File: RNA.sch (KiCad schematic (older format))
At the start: 89 parts, among them J1 USB_B_Micro, J2 AudioJack4, J3 AudioJack4, J4 Conn_01x06, SW1 SW_SPST, SW10 SW_Push_45deg, SW11 SW_Push_45deg, SW12 SW_Push_45deg, SW13 SW_Push_45deg, SW14 SW_Push_45deg, SW15 SW_Push_45deg, SW16 SW_Push_45deg, SW17 SW_Push_45deg, SW18 SW_Push_45deg, SW19 SW_Push_45deg, SW2 SW_Push, SW20 SW_Push_45deg, SW21 SW_Push_45deg, SW22 SW_Push_45deg, SW23 SW_Push_45deg, SW24 SW_Push_45deg, SW25 SW_Push_45deg, SW26 SW_Push_45deg, SW27 SW_Push_45deg, SW28 SW_Push_45deg, SW29 SW_Push_45deg, SW3 SW_Push_45deg, SW30 SW_Push_45deg, SW31 SW_Push_45deg, SW32 SW_Push_45deg, SW33 SW_Push_45deg, SW34 SW_Push_45deg, SW4 SW_Push_45deg, SW5 SW_Push_45deg, SW6 SW_Push_45deg, SW7 SW_Push_45deg, SW8 SW_Push_45deg, SW9 SW_Push_45deg, U1 STM32F072C8Tx, U2 PRTR5V0U2X, U3 MCP1703A-3302_SOT23, U4 CAT24M01W

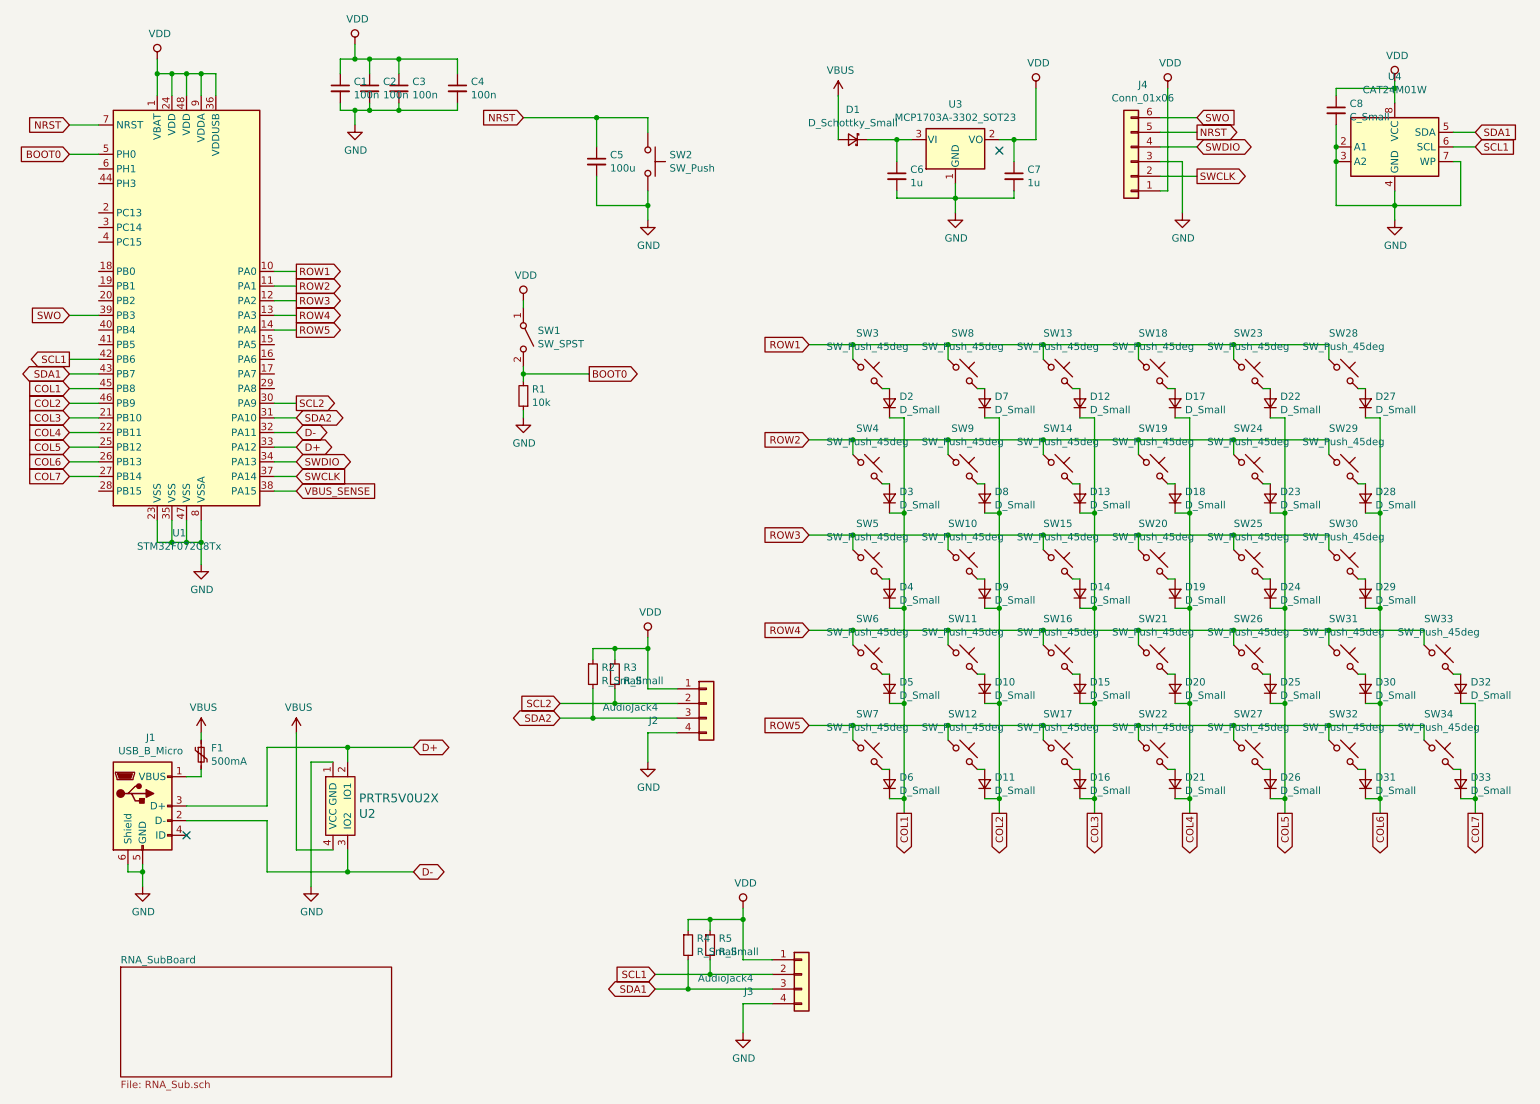
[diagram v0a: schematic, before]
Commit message: modify module
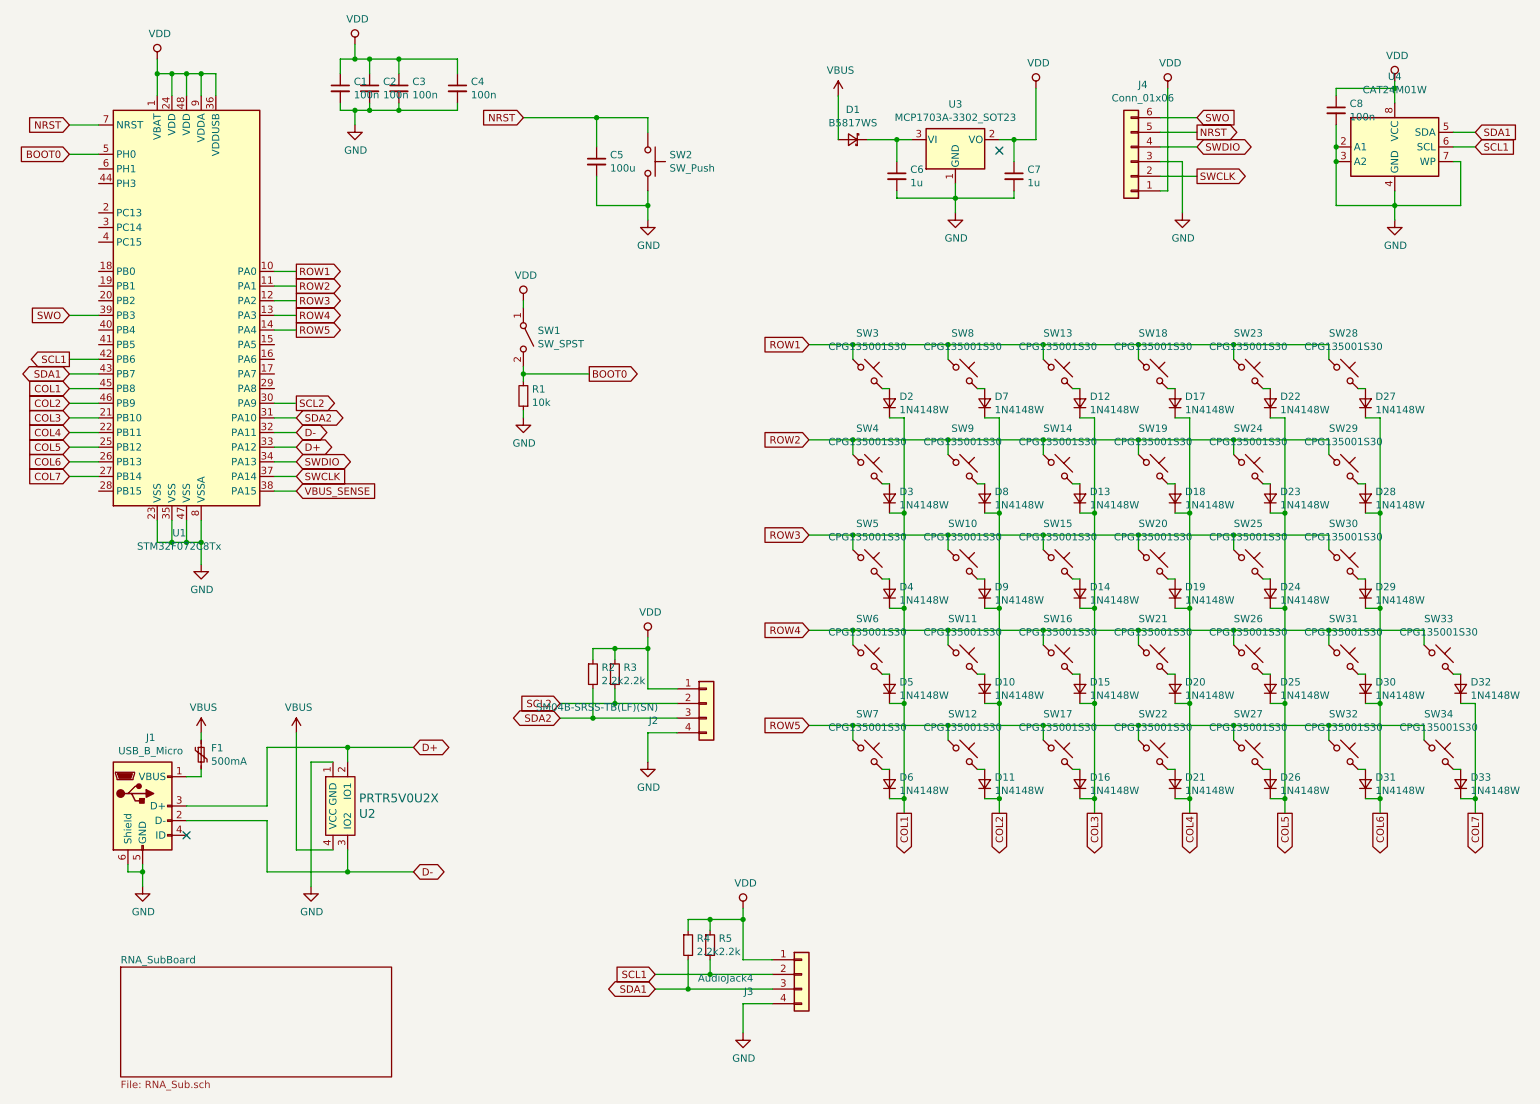
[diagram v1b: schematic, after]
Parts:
- C8: value C_Small -> 100n
- D1: value D_Schottky_Small -> B5817WS
- D10, D11, D12, D13, D14, D15, D16, D17, D18, D19, D2, D20, D21, D22, D23, D24, D25, D26, D27, D28, D29, D3, D30, D31, D32, D33, D4, D5, D6, D7, D8, D9: value D_Small -> 1N4148W
- J2: value AudioJack4 -> SM04B-SRSS-TB(LF)(SN)
- R2, R3, R4, R5: value R_Small -> 2.2k
- SW10, SW11, SW12, SW13, SW14, SW15, SW16, SW17, SW18, SW19, SW20, SW21, SW22, SW23, SW24, SW25, SW26, SW27, SW28, SW29, SW3, SW30, SW31, SW32, SW33, SW34, SW4, SW5, SW6, SW7, SW8, SW9: value SW_Push_45deg -> CPG135001S30
